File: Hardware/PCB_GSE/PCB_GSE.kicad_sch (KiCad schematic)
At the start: 36 parts, among them J1 Conn_01x06_Pin, U1 STM32F103CBT6

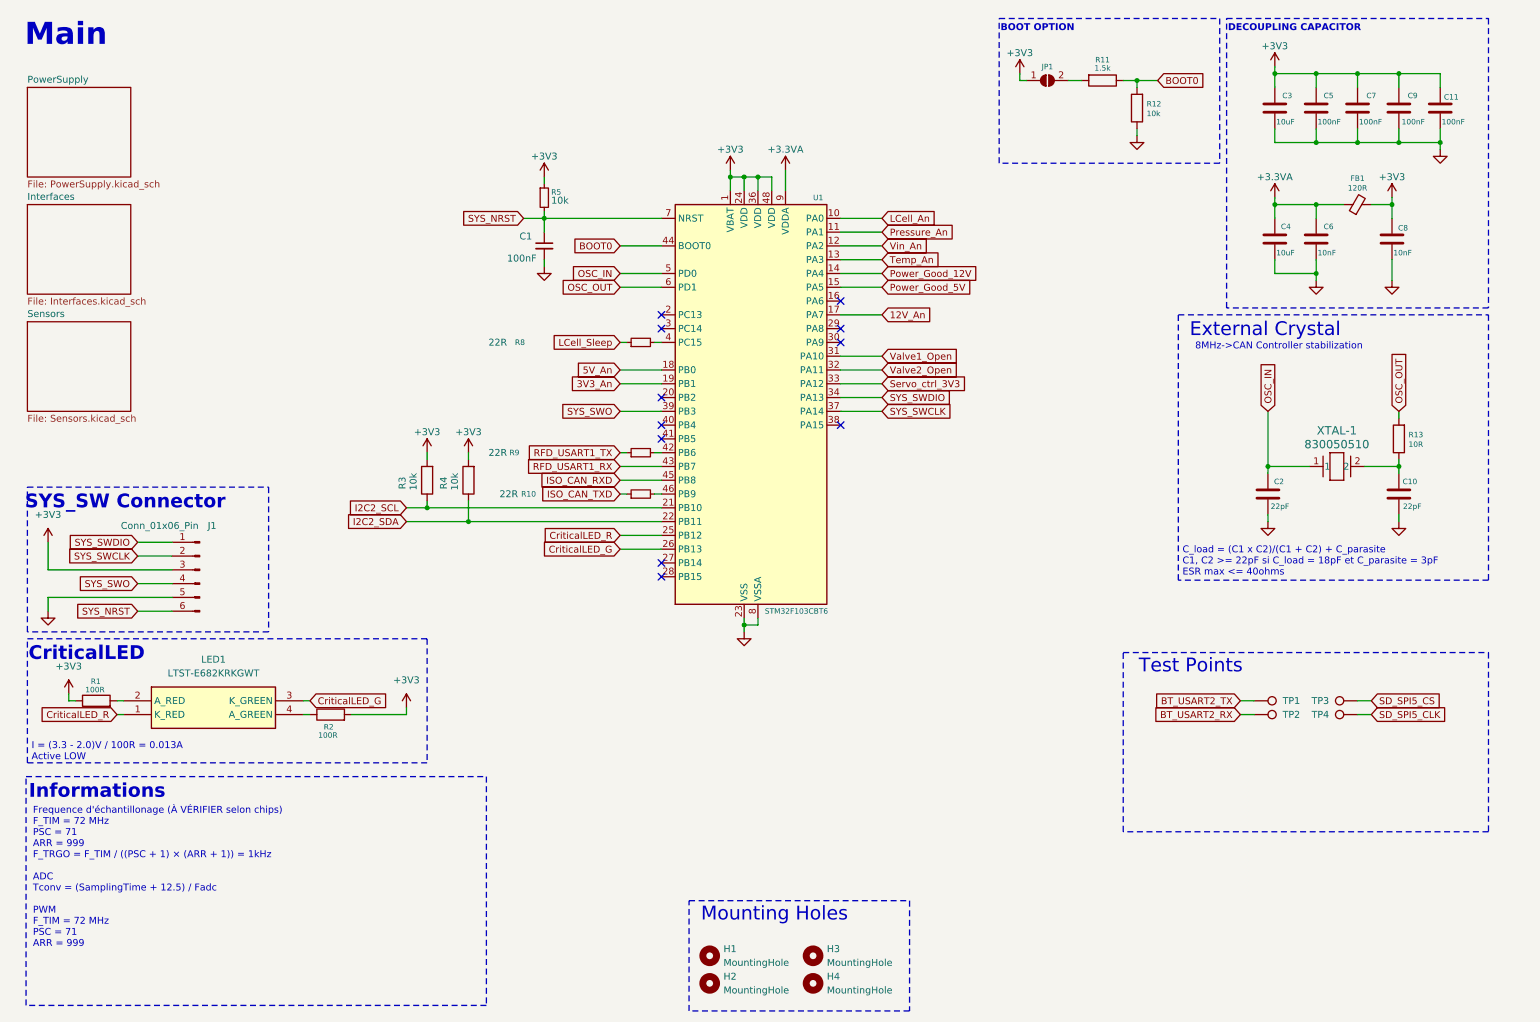
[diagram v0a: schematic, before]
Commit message: fix : done silkscreen and finition
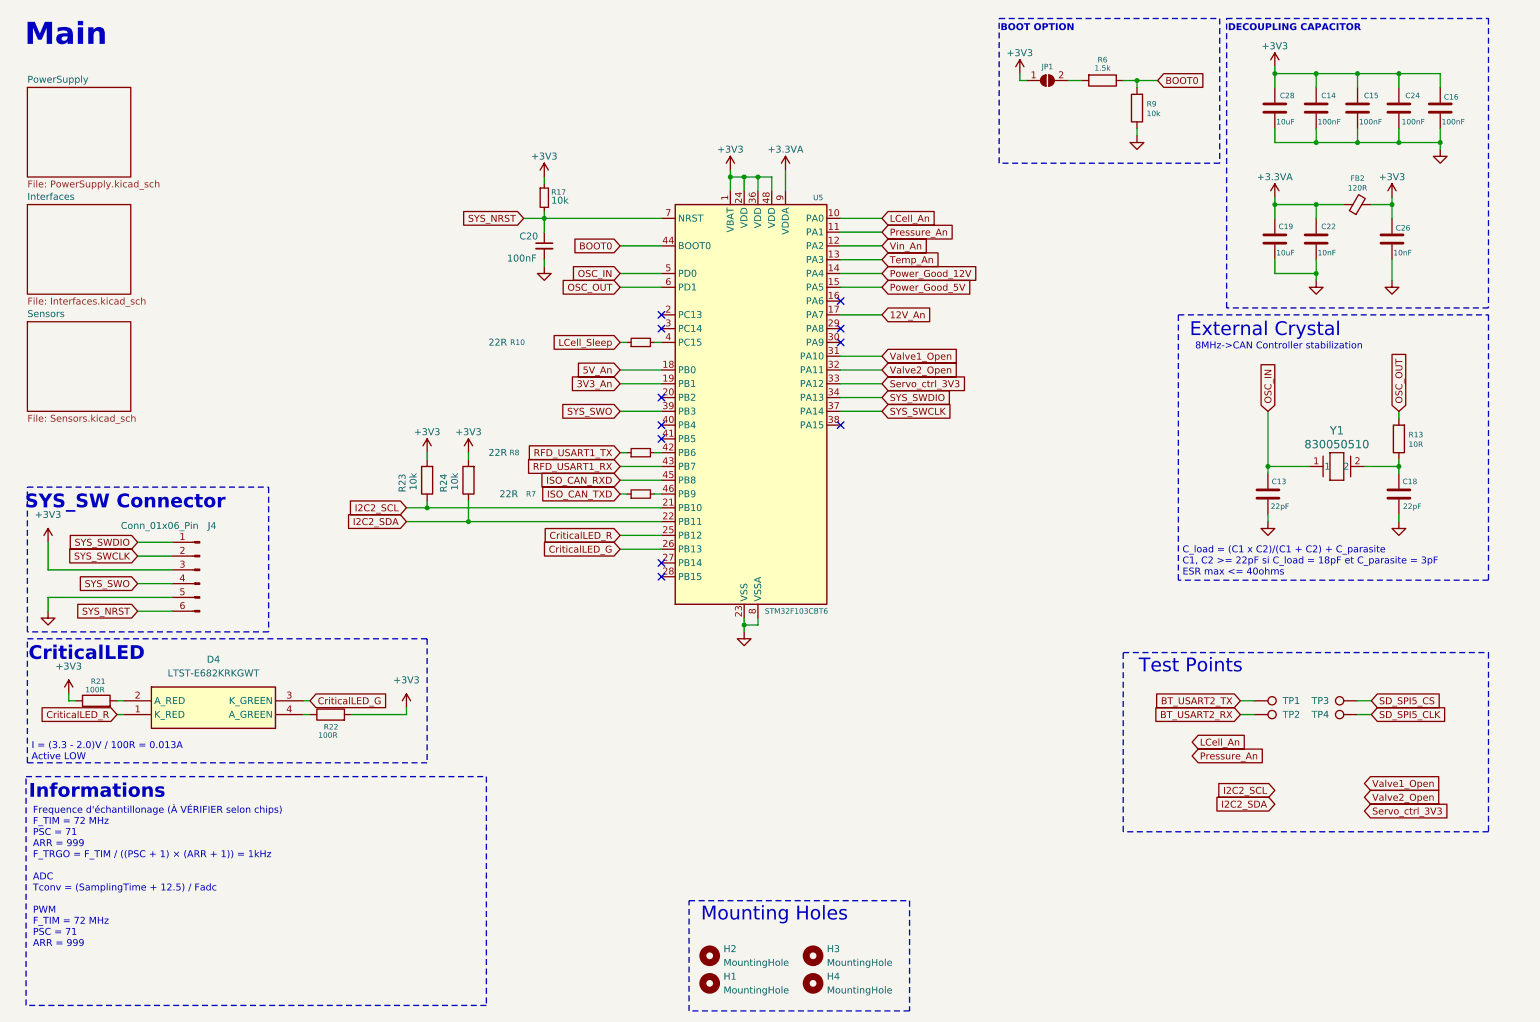
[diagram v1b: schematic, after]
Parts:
- renumbered C2 to C13, C5 to C14, C7 to C15, C11 to C16, C10 to C18, C4 to C19, C1 to C20, C6 to C22, C9 to C24, C8 to C26, C3 to C28, LED1 to D4, FB1 to FB2, H2 to H1, H1 to H2, J1 to J4, R8 to R10, R5 to R17, R1 to R21, R2 to R22, R3 to R23, R4 to R24, R11 to R6, R10 to R7, R9 to R8, R12 to R9, U1 to U5, XTAL-1 to Y1
